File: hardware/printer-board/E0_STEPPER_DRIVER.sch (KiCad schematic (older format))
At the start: 9 parts, among them J15 MS_SELECT, J16 E0, U9 A4988_MODULE

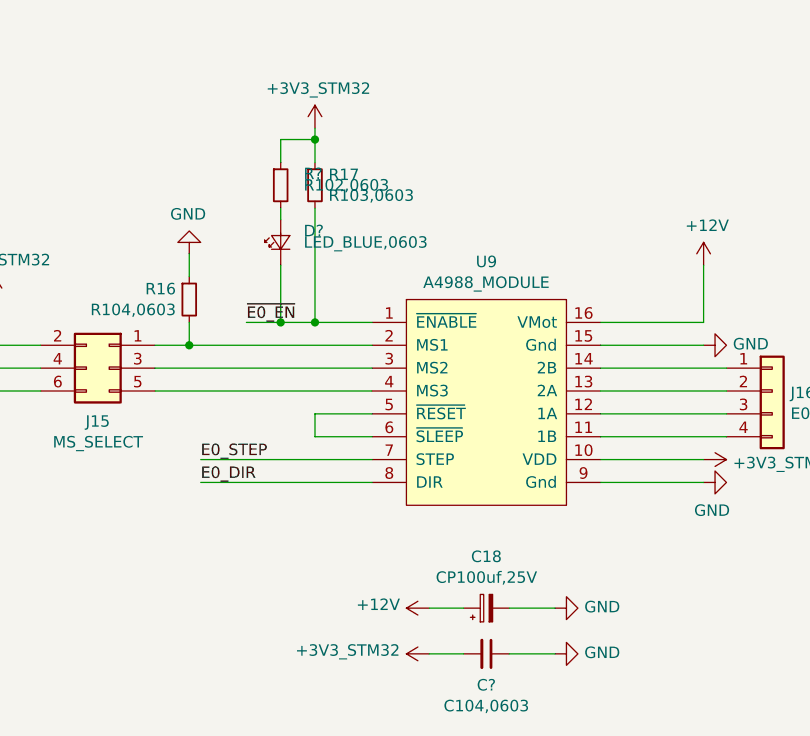
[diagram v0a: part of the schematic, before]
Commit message: update annotations,
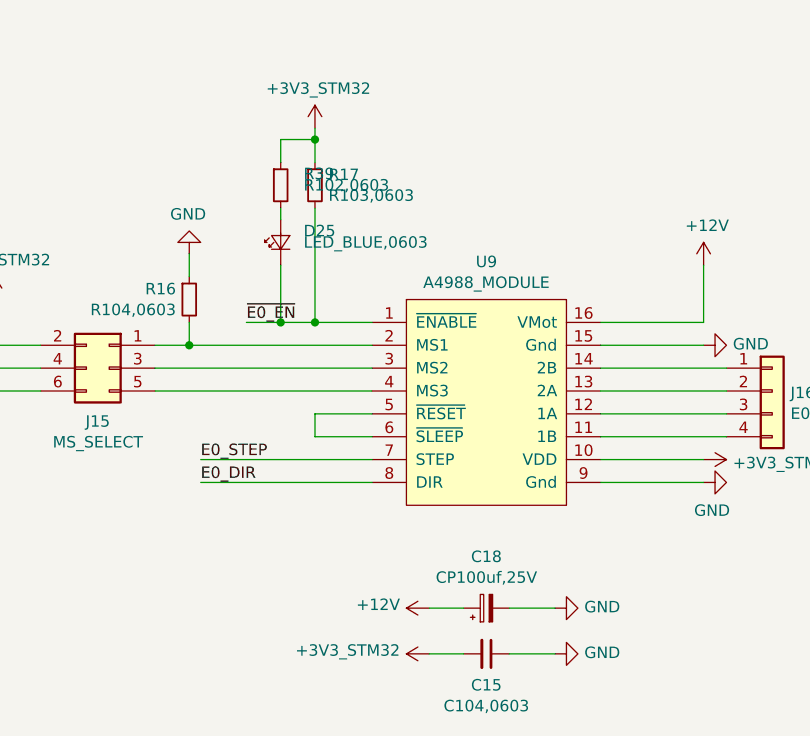
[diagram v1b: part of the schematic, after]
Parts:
- gave numbers to parts that had none: 3
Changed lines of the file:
@@
 $EndBitmap
 $Comp
-L taobao-components:+3V3_STM32 #PWR?
+L taobao-components:+3V3_STM32 #PWR026
 U 1 1 5CC8CD5D
 P 4900 1950
-F 0 "#PWR?" H 4900 1800 50  0001 C CNN
+F 0 "#PWR026" H 4900 1800 50  0001 C CNN
 F 1 "+3V3_STM32" H 4915 2123 50  0000 C CNN
 F 2 "" H 4900 1950 50  0001 C CNN
@@
 $EndComp
 $Comp
-L taobao-components:+3V3_STM32 #PWR?
+L taobao-components:+3V3_STM32 #PWR027
 U 1 1 5CC8CDB8
 P 3500 2700
-F 0 "#PWR?" H 3500 2550 50  0001 C CNN
+F 0 "#PWR027" H 3500 2550 50  0001 C CNN
 F 1 "+3V3_STM32" H 3515 2873 50  0000 C CNN
 F 2 "" H 3500 2700 50  0001 C CNN
@@
 $EndComp
 $Comp
-L taobao-components:+3V3_STM32 #PWR?
+L taobao-components:+3V3_STM32 #PWR028
 U 1 1 5CC8CEC9
 P 6600 3400
-F 0 "#PWR?" H 6600 3250 50  0001 C CNN
+F 0 "#PWR028" H 6600 3250 50  0001 C CNN
 F 1 "+3V3_STM32" V 6615 3528 50  0000 L CNN
 F 2 "" H 6600 3400 50  0001 C CNN
@@
 $EndComp
 $Comp
-L taobao-components:+3V3_STM32 #PWR?
+L taobao-components:+3V3_STM32 #PWR029
 U 1 1 5CC8DC63
 P 5400 4250
-F 0 "#PWR?" H 5400 4100 50  0001 C CNN
+F 0 "#PWR029" H 5400 4100 50  0001 C CNN
 F 1 "+3V3_STM32" V 5415 4378 50  0000 L CNN
 F 2 "" H 5400 4250 50  0001 C CNN
@@
 $EndComp
 $Comp
-L taobao-c:C104,0603 C?
+L taobao-c:C104,0603 C15
 U 1 1 5CC8EC71
 P 5650 4250
-F 0 "C?" V 5787 4250 50  0000 C CNN
+F 0 "C15" V 5787 4250 50  0000 C CNN
 F 1 "C104,0603" V 5878 4250 50  0000 C CNN
 F 2 "Capacitor_SMD:C_0603_1608Metric_Pad1.05x0.95mm_HandSolder" H 5650 4250 50  0001 C CNN
@@
 P 4750 2200
 AR Path="/5CC15C35/5CC4C25E" Ref="R?"  Part="1"
-AR Path="/5CC0AEC9/5CC4C25E" Ref="R?"  Part="1"
-F 0 "R?" H 4850 2250 50  0000 L CNN
+AR Path="/5CC0AEC9/5CC4C25E" Ref="R39"  Part="1"
+F 0 "R39" H 4850 2250 50  0000 L CNN
 F 1 "R102,0603" H 4850 2200 50  0000 L CNN
 F 2 "Resistor_SMD:R_0603_1608Metric_Pad1.05x0.95mm_HandSolder" H 4750 2200 50  0001 C CNN
@@
 P 4750 2450
 AR Path="/5CC15C35/5CC4C265" Ref="D?"  Part="1"
-AR Path="/5CC0AEC9/5CC4C265" Ref="D?"  Part="1"
-F 0 "D?" V 4800 2350 50  0000 R CNN
+AR Path="/5CC0AEC9/5CC4C265" Ref="D25"  Part="1"
+F 0 "D25" V 4800 2350 50  0000 R CNN
 F 1 "LED_BLUE,0603" V 4750 2350 50  0000 R CNN
 F 2 "LED_SMD:LED_0603_1608Metric_Pad1.05x0.95mm_HandSolder" V 4750 2450 50  0001 C CNN

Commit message: update,
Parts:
- J16: footprint footprint-lib:s4b-ph-kl,stepper_motor_terminal -> footprint-lib:b4b-ph-kl,stepper_terminal
- U9: footprint Module:Pololu_Breakout-16_15.2x20.3mm -> footprint-lib:Pololu_Breakout-16_15.2x20.3mm
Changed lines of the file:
@@
 $Descr A4 11693 8268
 encoding utf-8
-Sheet 10 33
+Sheet 7 33
 Title ""
 Date ""
@@
 F 0 "U9" H 5650 3765 50  0000 C CNN
 F 1 "A4988_MODULE" H 5650 3674 50  0000 C CNN
-F 2 "Module:Pololu_Breakout-16_15.2x20.3mm" H 5650 3200 50  0001 C CNN
+F 2 "footprint-lib:Pololu_Breakout-16_15.2x20.3mm" H 5650 3200 50  0001 C CNN
 F 3 "" H 5650 3200 50  0001 C CNN
 	1    5650 3150
@@
 F 0 "J16" H 6980 3092 50  0000 L CNN
 F 1 "E0" H 6980 3001 50  0000 L CNN
-F 2 "footprint-lib:s4b-ph-kl,stepper_motor_terminal" H 6900 3100 50  0001 C CNN
+F 2 "footprint-lib:b4b-ph-kl,stepper_terminal" H 6900 3100 50  0001 C CNN
 F 3 "~" H 6900 3100 50  0001 C CNN
 	1    6900 3100
